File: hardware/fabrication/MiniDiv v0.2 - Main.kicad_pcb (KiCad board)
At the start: 2 copper layers, 65 x 128.5 mm, 85 parts, among them J1 Conn_01x10_Pin, SW1 SW_DPDT_x2, U1 40106, U2 LM358, U3 40106, U4 LM317_SOT-223, U5 CD4040

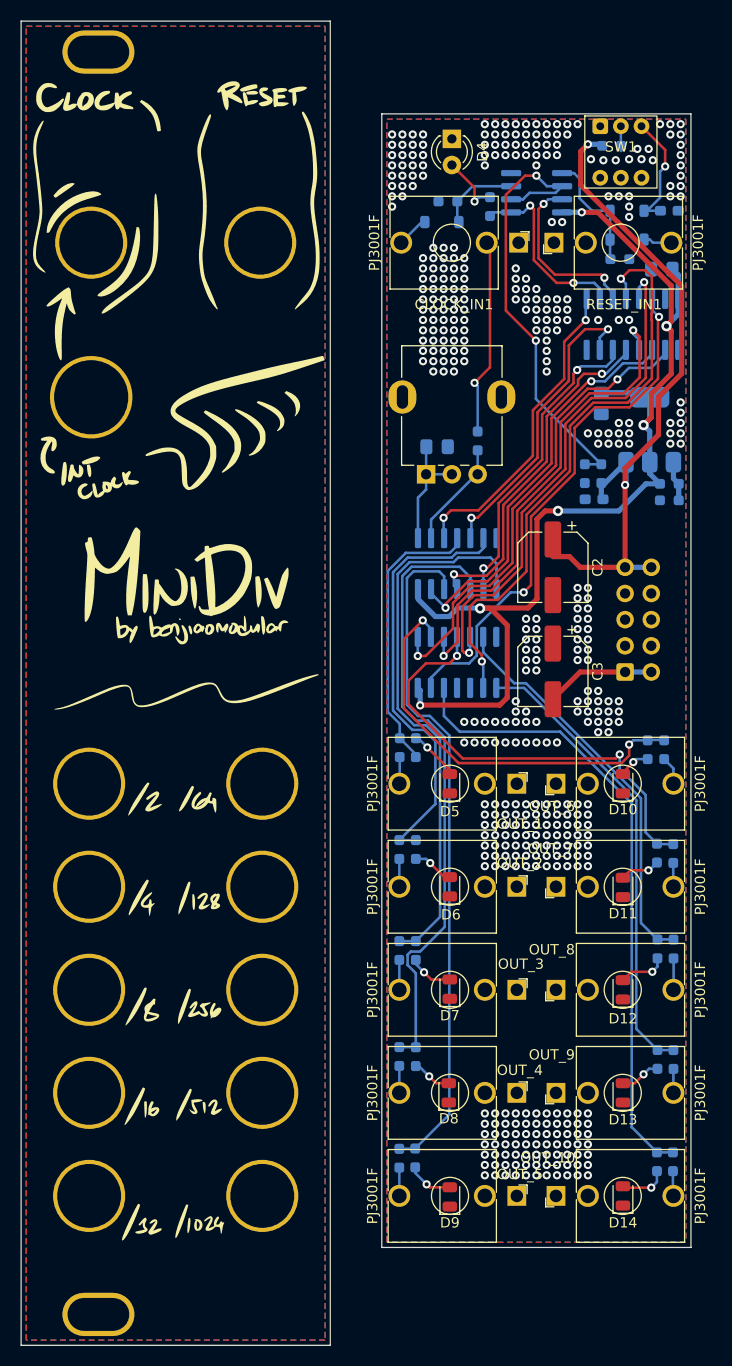
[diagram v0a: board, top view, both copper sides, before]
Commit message: v0.2 PCB
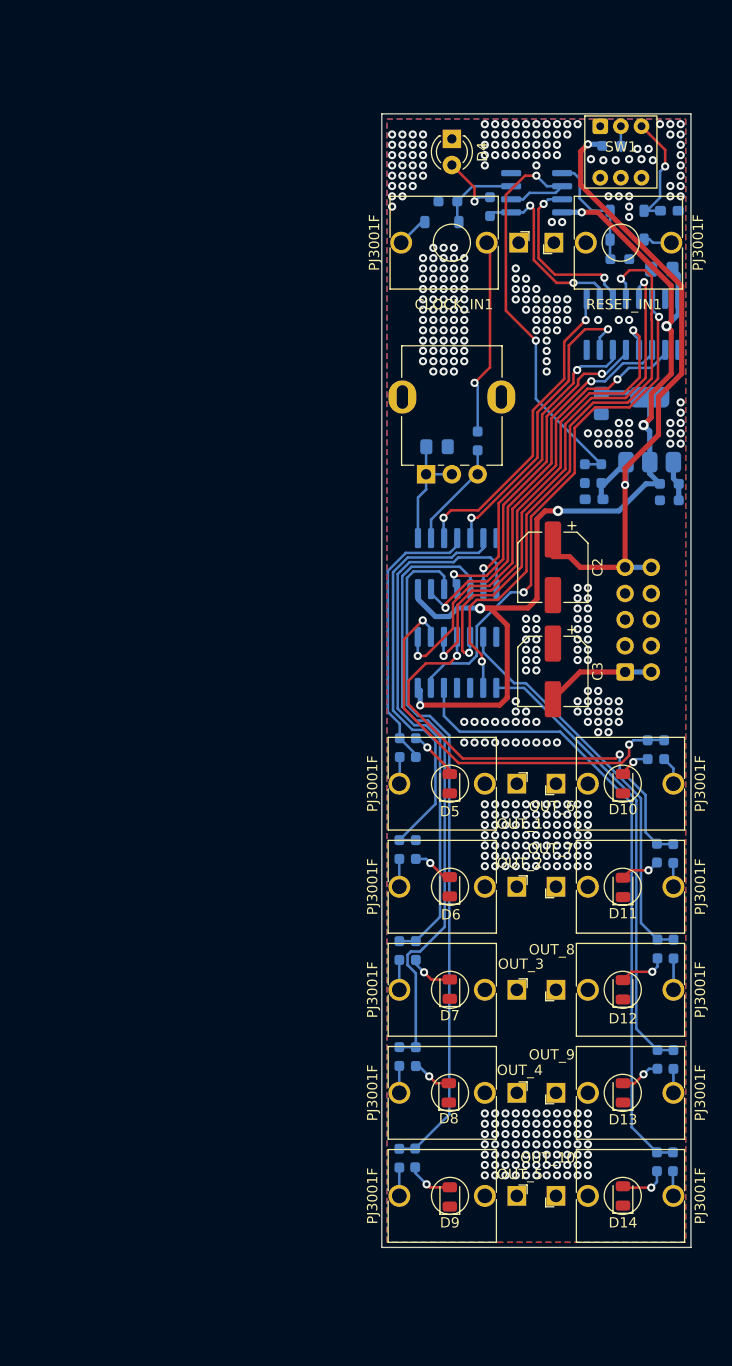
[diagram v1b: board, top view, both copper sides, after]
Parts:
- removed G***: LOGO, LOGO
- removed REF** (x12): PanelHole_AudioJack_3.5mm, benjiaomodular:PanelHole_AudioJack_3.5mm
- removed REF**: Panel_6HP, benjiaomodular:Panel_6HP
- removed REF**: PanelHole_Potentiometer_RV09, benjiaomodular:PanelHole_Potentiometer_RV09
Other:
- board size 65 x 128.5 mm -> 30 x 110 mm
